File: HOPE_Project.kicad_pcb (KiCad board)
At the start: 2 copper layers, 114.7 x 113.4 mm, 26 parts, among them J1 Serial_to_USB, J2 LCD_Screen, U1 V7805-1000, U2 ATmega168A-PU, Y1 Crystal

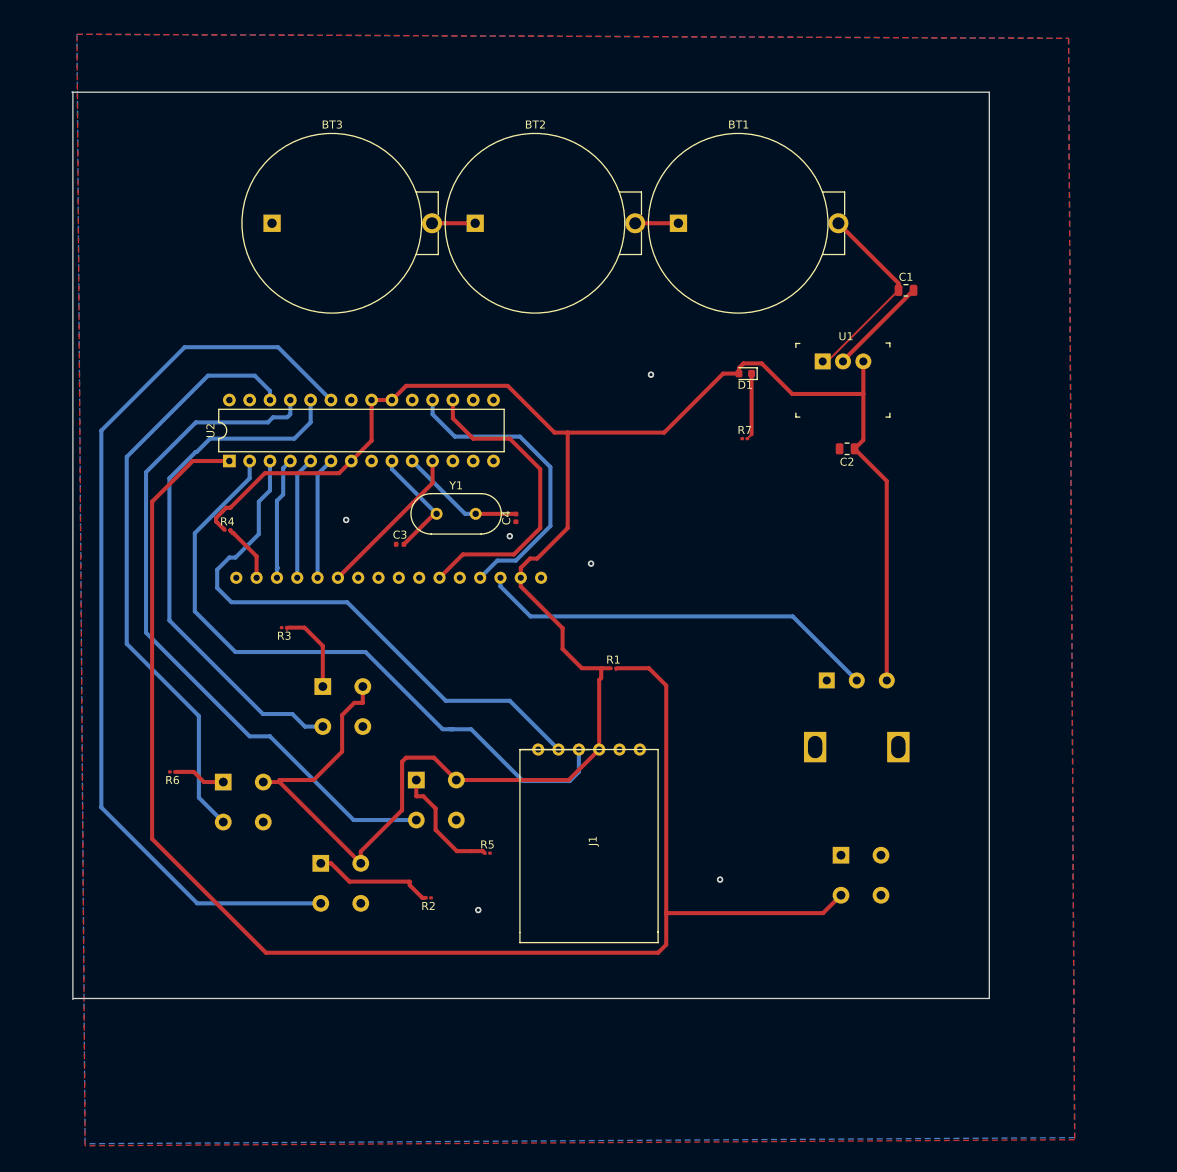
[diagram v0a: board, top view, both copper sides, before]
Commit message: First round of adjustments
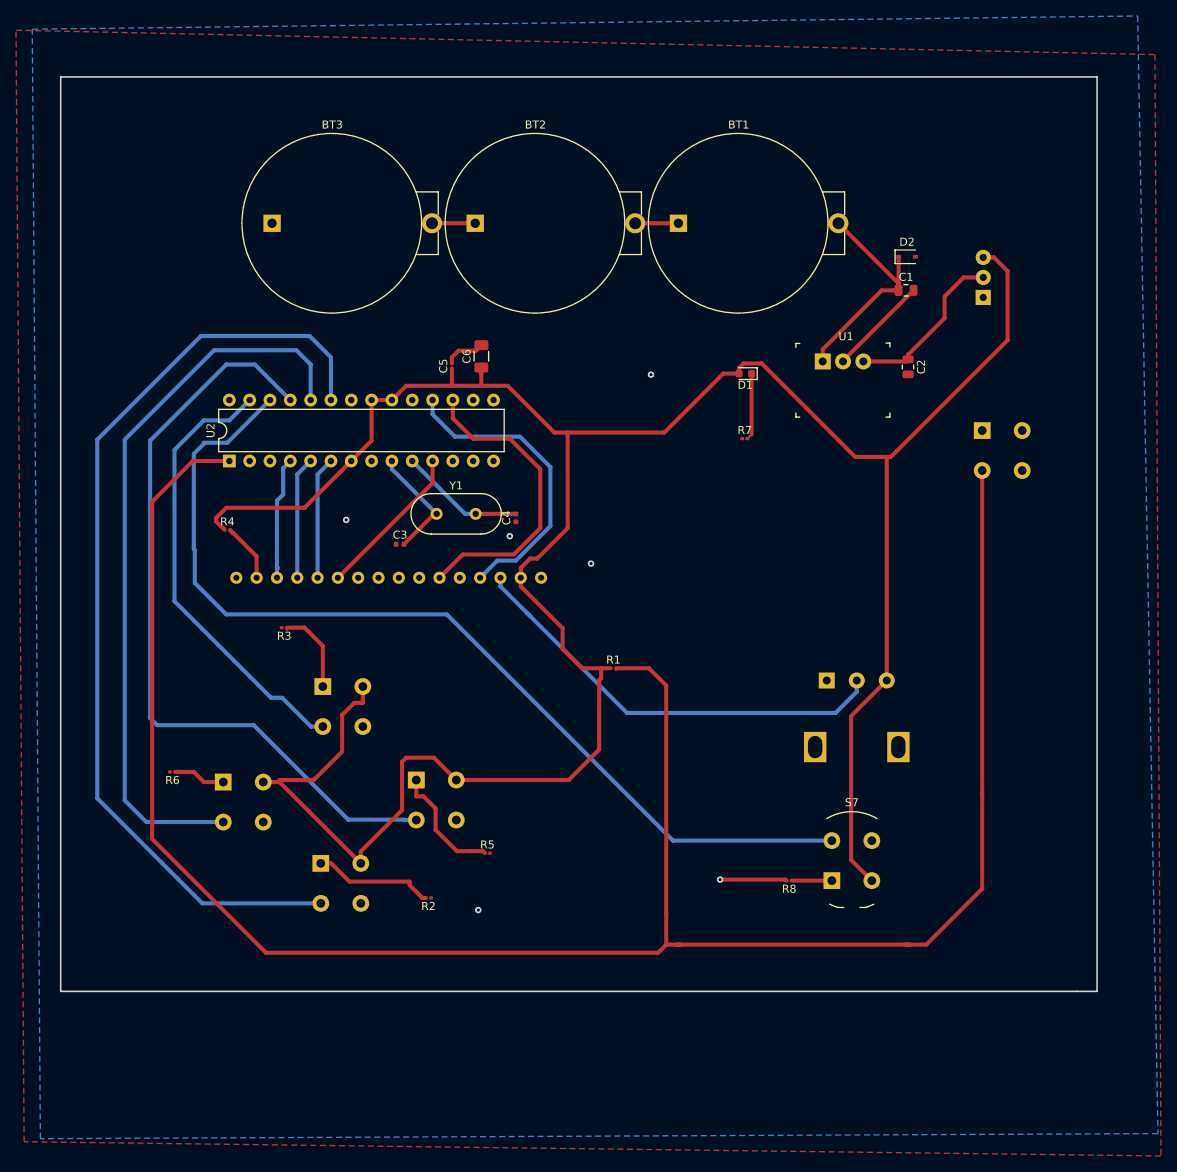
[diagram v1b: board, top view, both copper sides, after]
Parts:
- removed J1: Serial_to_USB, HOPE_Project:Serial_Breakout
- added C5: 100 nF, Capacitor_SMD:C_0201_0603Metric, F.Cu at (74.3, 84.4)
- added C6: 100 uF, Capacitor_SMD:C_1206_3216Metric, F.Cu at (78.0, 83.2)
- added D2: D_Schottky, Diode_SMD:D_SOD-323, F.Cu at (131.2, 70.7)
- added R8: 10 kOhm, Resistor_SMD:R_0201_0603Metric, F.Cu at (116.5, 148.7)
- added S6: EG1903-ND, digikey-footprints:Switch_Slide_11.6x4mm_EG1218, B.Cu at (140.7, 75.8)
- added S7: KS-01Q-01, digikey-footprints:PushButton_Round_D12mm_THT_KS-01Q-01, F.Cu at (121.8, 148.7)
- R2, R3, R5, R6: value 1 kOhm -> 10 kOhm
- moved S1 55.9 mm to (140.6, 92.5)
- moved C2 12.8 mm to (131.3, 84.5), turned to 270 degrees
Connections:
- C2 pad 1: +5V -> Net-(C2-Pad1)
- S3 pad 3: /A1 -> /A4
- S5 pad 3: /A3 -> /A1
- U1 pad 3: +5V -> Net-(C2-Pad1)
- U2 pad 2: /RX -> Net-(U2-Pad2)
- U2 pad 27: Net-(U2-Pad27) -> /A4
- U2 pad 3: /TX -> Net-(U2-Pad3)
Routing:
- net /RX: track 82.1 -> 0.00 mm
- net /RST_BTN: track 186.9 -> 259.7 mm
- net /TX: track 70.1 -> 0.00 mm
- net +5V: track 270.5 -> 328.9 mm
- net /A4: track 0.00 -> 55.9 mm
- net /A3: track 74.7 -> 121.5 mm
- net /A1: track 65.8 -> 91.6 mm
- net Net-(C2-Pad1): track 0.00 -> 21.3 mm
- net GND: track 12.5 -> 25.9 mm
- net /A2: track 86.4 -> 96.5 mm
- net Net-(BT1-Pad1): track 24.7 -> 30.3 mm
- net Net-(R8-Pad1): track 0.00 -> 5.01 mm
- net Net-(J2-Pad3): track 50.5 -> 55.3 mm
- net /A0: track 115.3 -> 119.2 mm
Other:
- board size 114.7 x 113.4 mm -> 129.5 x 114.3 mm
